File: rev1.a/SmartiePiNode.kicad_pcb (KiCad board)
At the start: 2 copper layers, 71.7 x 55 mm, 62 parts, among them CN1 USBMICROb, CN2 SWD, CN3 SX1238_TRX_HEADER, CN4 VIN, SW1 SW_PUSH, U1 ISL91127IR, U2 STM32L052_LQFP48, X1 abm10, X2 ABS25-32.768KHZ-6-T

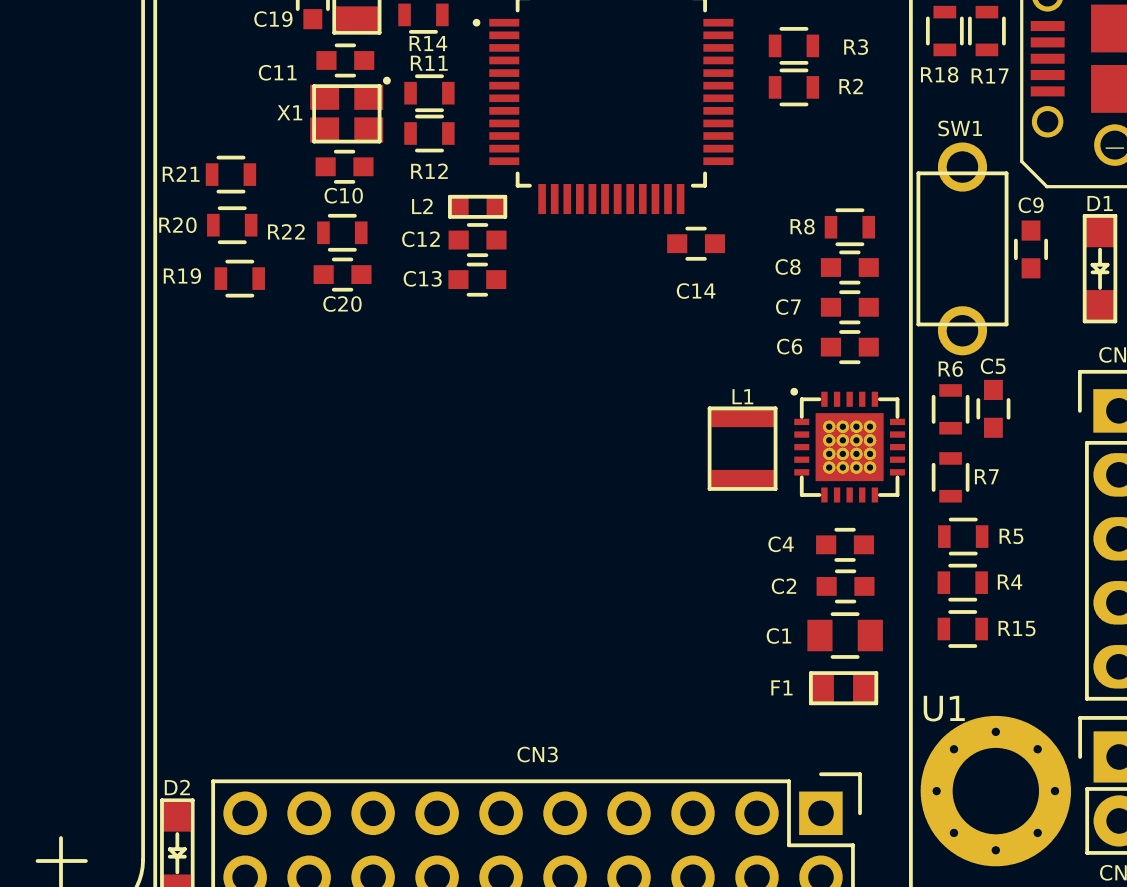
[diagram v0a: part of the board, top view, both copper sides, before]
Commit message: more pcb layout
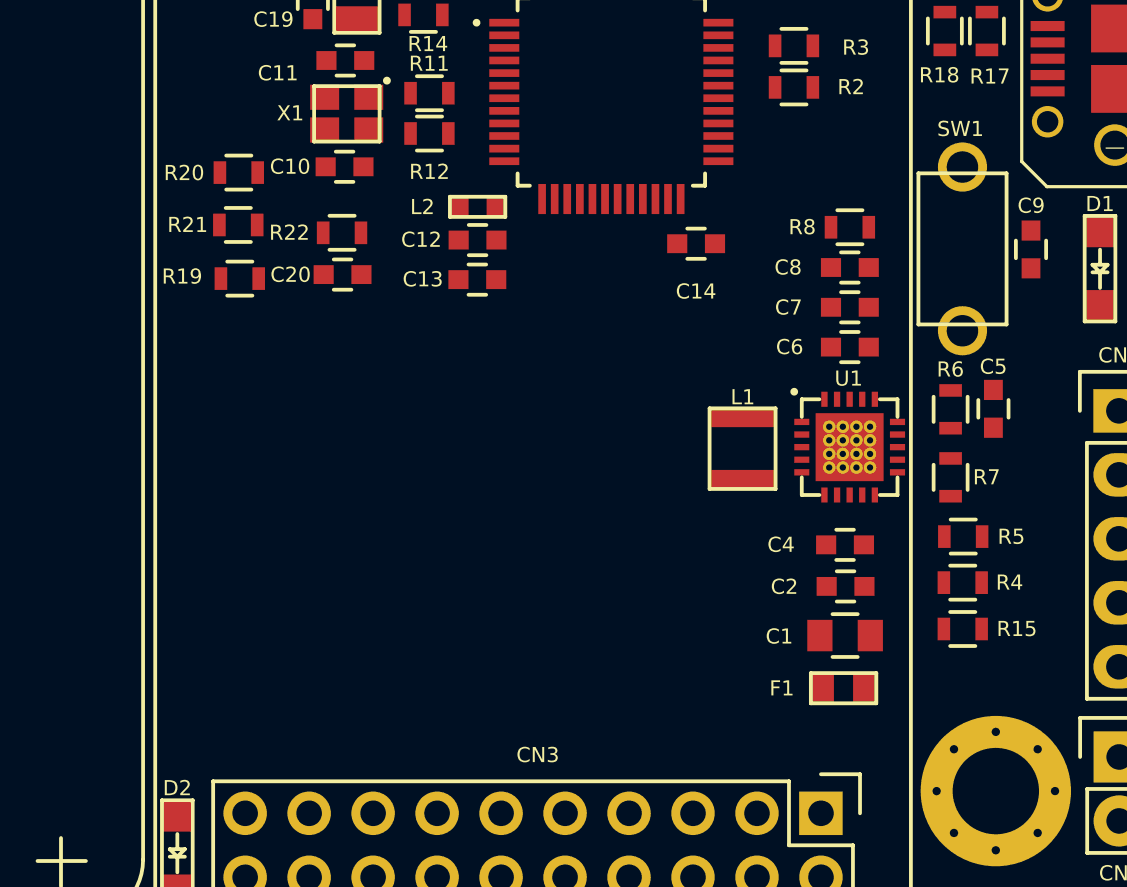
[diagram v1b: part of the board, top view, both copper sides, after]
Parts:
- moved R20 2.11 mm to (133.9, 120.4)
- moved R21 2.02 mm to (133.8, 122.4), turned to 0 degrees
- turned R22 to 180 degrees
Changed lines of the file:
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@@
     (tags "capacitor 0603")
     (attr smd)
-    (fp_text reference C10 (at 0.03 -1.17 180) (layer F.SilkS)
+    (fp_text reference C10 (at 2.16 0 180) (layer F.SilkS)
       (effects (font (size 0.6 0.6) (thickness 0.1)))
     )
@@
     (tags "capacitor 0603")
     (attr smd)
-    (fp_text reference C20 (at 0 1.19) (layer F.SilkS)
+    (fp_text reference C20 (at -2.06 0.01) (layer F.SilkS)
       (effects (font (size 0.6 0.6) (thickness 0.1)))
     )
@@
   )
   (module Resistors_SMD:R_0603 (layer F.Cu)
-    (at 133.6 122.45 180)
+    (at 133.86 120.36 180)
     (descr "Resistor SMD 0603, reflow soldering, Vishay (see dcrcw.pdf)")
     (tags "resistor 0603")
@@
   )
   (module Resistors_SMD:R_0603 (layer F.Cu)
-    (at 133.55 120.44 180)
-    (descr "Resistor SMD 0603, reflow soldering, Vishay (see dcrcw.pdf)")
-    (tags "resistor 0603")
-    (attr smd)
-    (fp_text reference R21 (at 1.98 -0.01 180) (layer F.SilkS)
+    (at 133.84 122.44)
+    (descr "Resistor SMD 0603, reflow soldering, Vishay (see dcrcw.pdf)")
+    (tags "resistor 0603")
+    (attr smd)
+    (fp_text reference R21 (at -2.01 0) (layer F.SilkS)
+      (effects (font (size 0.6 0.6) (thickness 0.1)))
+    )
+    (fp_text value DNP (at 0 1.9) (layer F.Fab)
+      (effects (font (size 0.6 0.6) (thickness 0.1)))
+    )
+    (fp_line (start -0.5 -0.675) (end 0.5 -0.675) (layer F.SilkS) (width 0.15))
+    (fp_line (start 0.5 0.675) (end -0.5 0.675) (layer F.SilkS) (width 0.15))
+    (fp_line (start 1.3 -0.8) (end 1.3 0.8) (layer F.CrtYd) (width 0.05))
+    (fp_line (start -1.3 -0.8) (end -1.3 0.8) (layer F.CrtYd) (width 0.05))
+    (fp_line (start -1.3 0.8) (end 1.3 0.8) (layer F.CrtYd) (width 0.05))
+    (fp_line (start -1.3 -0.8) (end 1.3 -0.8) (layer F.CrtYd) (width 0.05))
+    (pad 2 smd rect (at 0.75 0) (size 0.5 0.9) (layers F.Cu F.Paste F.Mask)
+      (net 77 /VSENSE))
+    (pad 1 smd rect (at -0.75 0) (size 0.5 0.9) (layers F.Cu F.Paste F.Mask)
+      (net 76 "Net-(R19-Pad2)"))
+    (model Resistors_SMD.3dshapes/R_0603.wrl
+      (at (xyz 0 0 0))
+      (scale (xyz 1 1 1))
+      (rotate (xyz 0 0 0))
+    )
+  )
+  (module Resistors_SMD:R_0603 (layer F.Cu)
+    (at 137.96 122.75 180)
+    (descr "Resistor SMD 0603, reflow soldering, Vishay (see dcrcw.pdf)")
+    (tags "resistor 0603")
+    (attr smd)
+    (fp_text reference R22 (at 2.09 0 180) (layer F.SilkS)
       (effects (font (size 0.6 0.6) (thickness 0.1)))
     )
@@
       (effects (font (size 0.6 0.6) (thickness 0.1)))
     )
-    (fp_line (start -0.5 -0.675) (end 0.5 -0.675) (layer F.SilkS) (width 0.15))
-    (fp_line (start 0.5 0.675) (end -0.5 0.675) (layer F.SilkS) (width 0.15))
-    (fp_line (start 1.3 -0.8) (end 1.3 0.8) (layer F.CrtYd) (width 0.05))
-    (fp_line (start -1.3 -0.8) (end -1.3 0.8) (layer F.CrtYd) (width 0.05))
-    (fp_line (start -1.3 0.8) (end 1.3 0.8) (layer F.CrtYd) (width 0.05))
-    (fp_line (start -1.3 -0.8) (end 1.3 -0.8) (layer F.CrtYd) (width 0.05))
+    (fp_line (start -1.3 -0.8) (end 1.3 -0.8) (layer F.CrtYd) (width 0.05))
+    (fp_line (start -1.3 0.8) (end 1.3 0.8) (layer F.CrtYd) (width 0.05))
+    (fp_line (start -1.3 -0.8) (end -1.3 0.8) (layer F.CrtYd) (width 0.05))
+    (fp_line (start 1.3 -0.8) (end 1.3 0.8) (layer F.CrtYd) (width 0.05))
+    (fp_line (start 0.5 0.675) (end -0.5 0.675) (layer F.SilkS) (width 0.15))
+    (fp_line (start -0.5 -0.675) (end 0.5 -0.675) (layer F.SilkS) (width 0.15))
+    (pad 1 smd rect (at -0.75 0 180) (size 0.5 0.9) (layers F.Cu F.Paste F.Mask)
+      (net 74 /VMEASURE))
     (pad 2 smd rect (at 0.75 0 180) (size 0.5 0.9) (layers F.Cu F.Paste F.Mask)
-      (net 77 /VSENSE))
-    (pad 1 smd rect (at -0.75 0 180) (size 0.5 0.9) (layers F.Cu F.Paste F.Mask)
-      (net 76 "Net-(R19-Pad2)"))
-    (model Resistors_SMD.3dshapes/R_0603.wrl
-      (at (xyz 0 0 0))
-      (scale (xyz 1 1 1))
-      (rotate (xyz 0 0 0))
-    )
-  )
-  (module Resistors_SMD:R_0603 (layer F.Cu)
-    (at 137.97 122.75)
-    (descr "Resistor SMD 0603, reflow soldering, Vishay (see dcrcw.pdf)")
-    (tags "resistor 0603")
-    (attr smd)
-    (fp_text reference R22 (at -2.22 -0.01) (layer F.SilkS)
-      (effects (font (size 0.6 0.6) (thickness 0.1)))
-    )
-    (fp_text value DNP (at 0 1.9) (layer F.Fab)
-      (effects (font (size 0.6 0.6) (thickness 0.1)))
-    )
-    (fp_line (start -1.3 -0.8) (end 1.3 -0.8) (layer F.CrtYd) (width 0.05))
-    (fp_line (start -1.3 0.8) (end 1.3 0.8) (layer F.CrtYd) (width 0.05))
-    (fp_line (start -1.3 -0.8) (end -1.3 0.8) (layer F.CrtYd) (width 0.05))
-    (fp_line (start 1.3 -0.8) (end 1.3 0.8) (layer F.CrtYd) (width 0.05))
-    (fp_line (start 0.5 0.675) (end -0.5 0.675) (layer F.SilkS) (width 0.15))
-    (fp_line (start -0.5 -0.675) (end 0.5 -0.675) (layer F.SilkS) (width 0.15))
-    (pad 1 smd rect (at -0.75 0) (size 0.5 0.9) (layers F.Cu F.Paste F.Mask)
-      (net 74 /VMEASURE))
-    (pad 2 smd rect (at 0.75 0) (size 0.5 0.9) (layers F.Cu F.Paste F.Mask)
       (net 76 "Net-(R19-Pad2)"))
     (model Resistors_SMD.3dshapes/R_0603.wrl
@@
   (module intersil-isl91127ir:intersil-isl91127ir (layer F.Cu)
     (at 158.11 131.26)
-    (fp_text reference U1 (at 3.76 10.41) (layer F.SilkS)
-      (effects (font (size 1 1) (thickness 0.15)))
+    (fp_text reference U1 (at -0.04 -2.72) (layer F.SilkS)
+      (effects (font (size 0.6 0.6) (thickness 0.1)))
     )
     (fp_text value ISL91127IR (at 3.75 -9.88) (layer F.Fab)
-      (effects (font (size 1 1) (thickness 0.15)))
+      (effects (font (size 0.6 0.6) (thickness 0.1)))
     )
     (fp_circle (center -2.2 -2.2) (end -2.15 -2.14) (layer F.SilkS) (width 0.15))

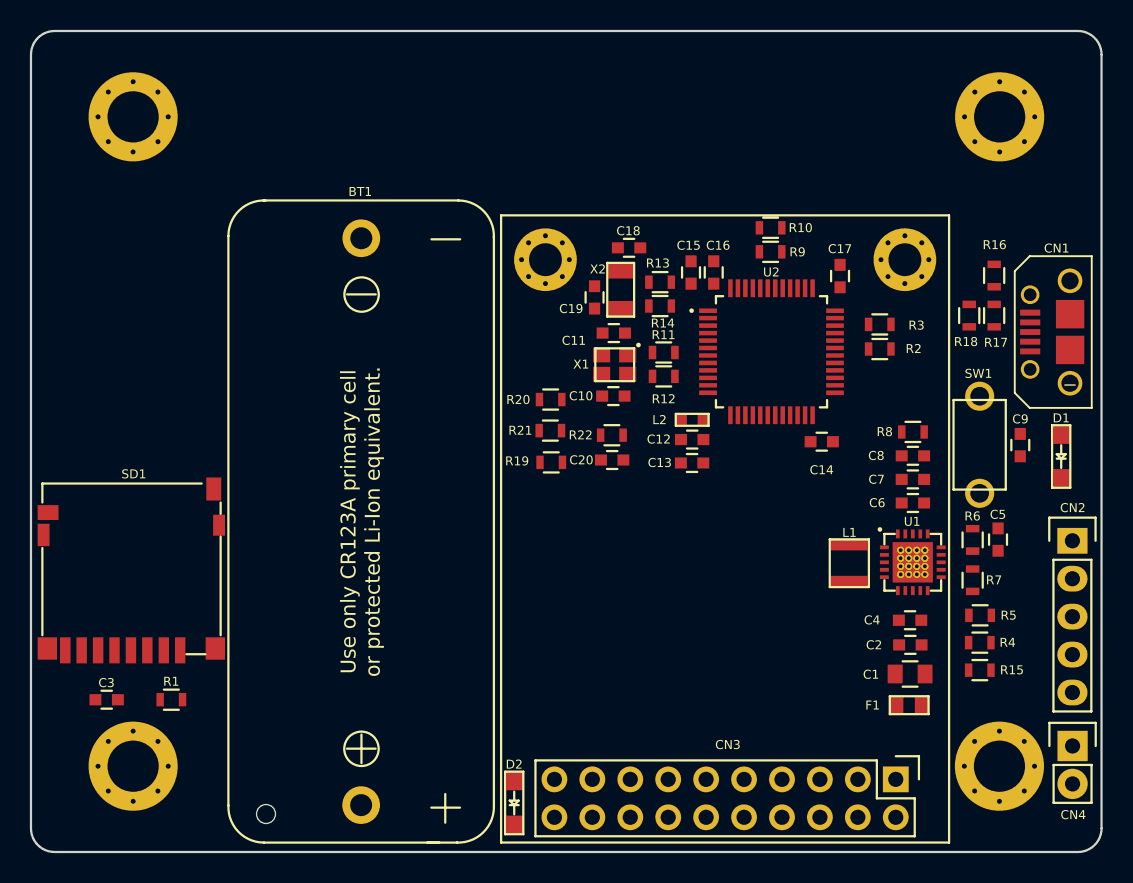
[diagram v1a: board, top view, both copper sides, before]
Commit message: finalizing layout
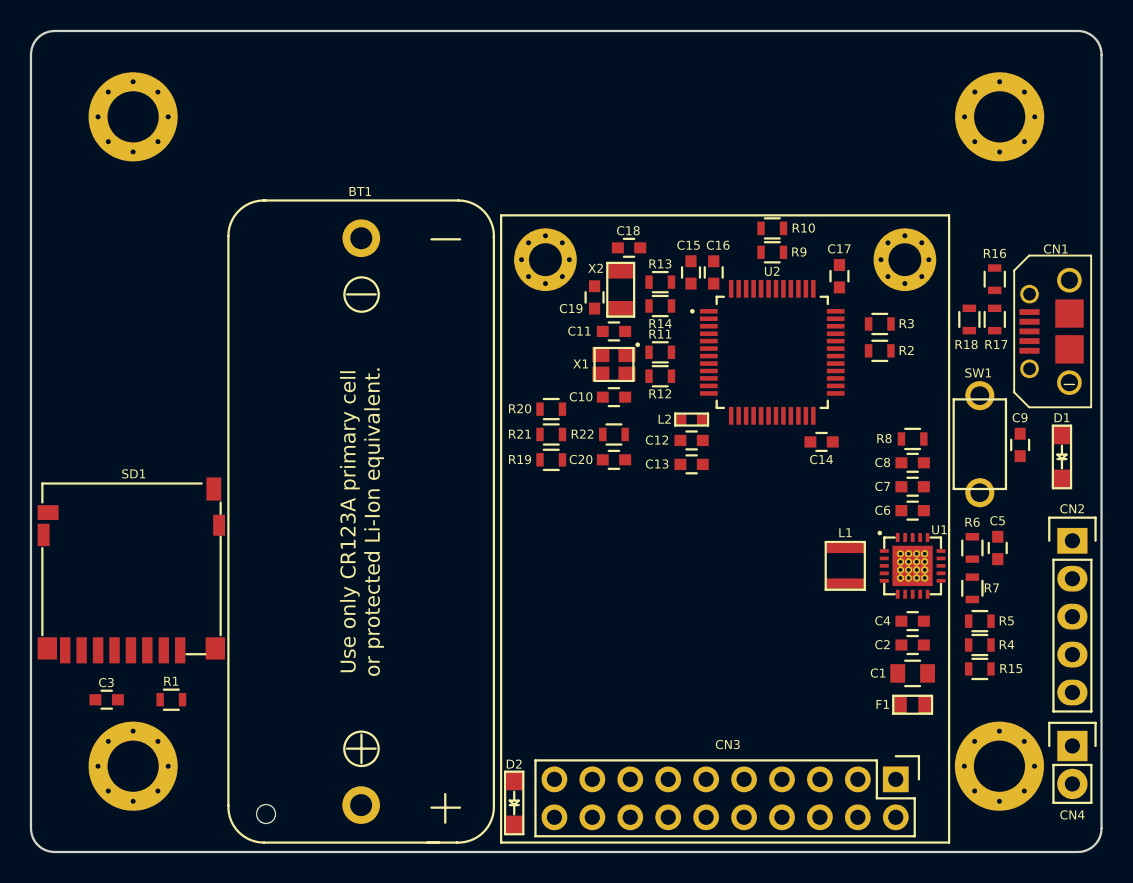
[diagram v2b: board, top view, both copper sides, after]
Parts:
- moved R20 0.64 mm to (133.9, 121.0)
- moved C5 0.56 mm to (163.8, 130.3)
- moved R6 0.54 mm to (162.1, 130.3)
- moved R7 0.54 mm to (162.1, 133.0)
- moved C6 0.51 mm to (158.1, 127.8)
- moved C7 0.49 mm to (158.1, 126.2)
- moved C8 0.47 mm to (158.1, 124.6)
- moved R8 0.47 mm to (158.1, 123.0)
- moved R5 0.39 mm to (162.6, 135.2)
- moved L1 0.32 mm to (153.6, 131.5)
- moved R21 0.27 mm to (133.9, 122.7)
- moved R17 0.26 mm to (163.6, 115.0)
- moved R18 0.26 mm to (161.9, 115.0)
- moved R16 0.24 mm to (163.6, 112.3)
- moved U1 0.24 mm to (158.1, 131.5)
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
